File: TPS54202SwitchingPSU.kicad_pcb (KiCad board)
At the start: 2 copper layers, 10 parts, among them CN1 Header_2_pin, CN2 Header_2_pin, U2 TPS54202DDC

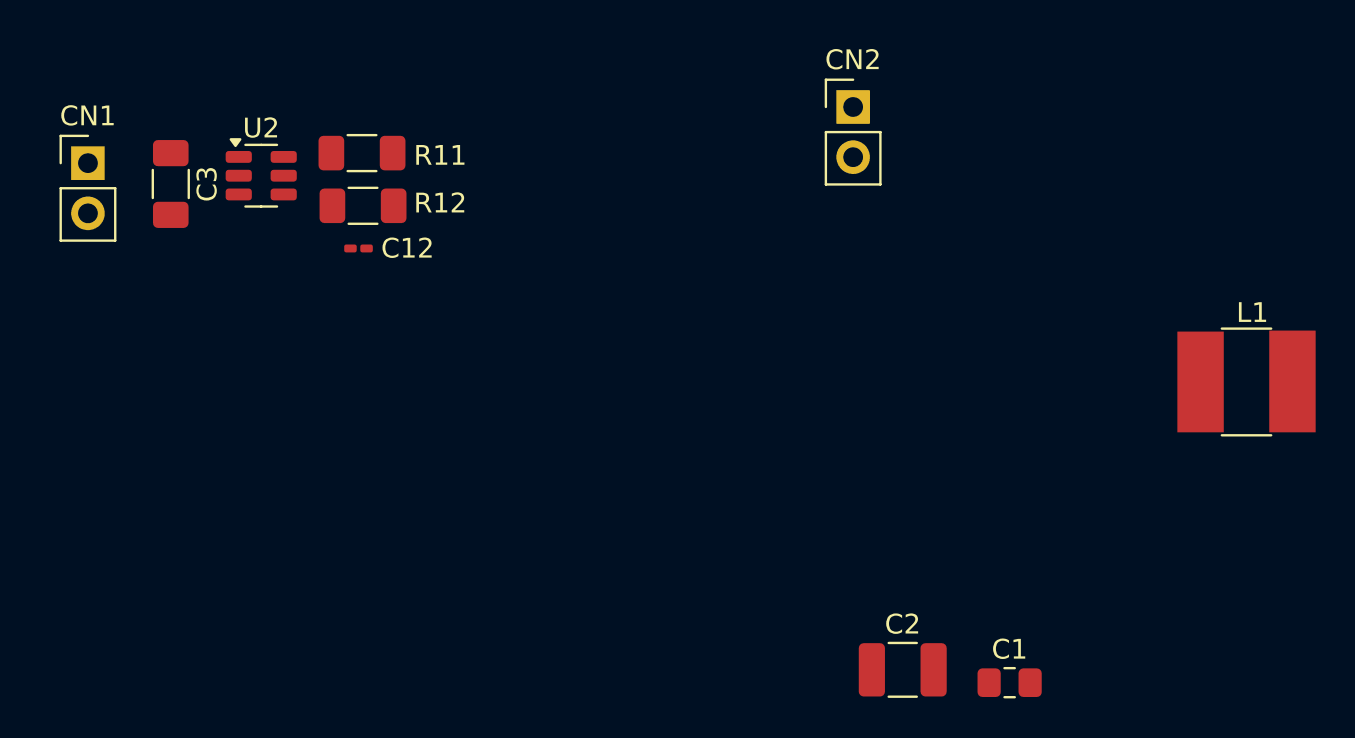
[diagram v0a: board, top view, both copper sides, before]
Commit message: Rev A production release
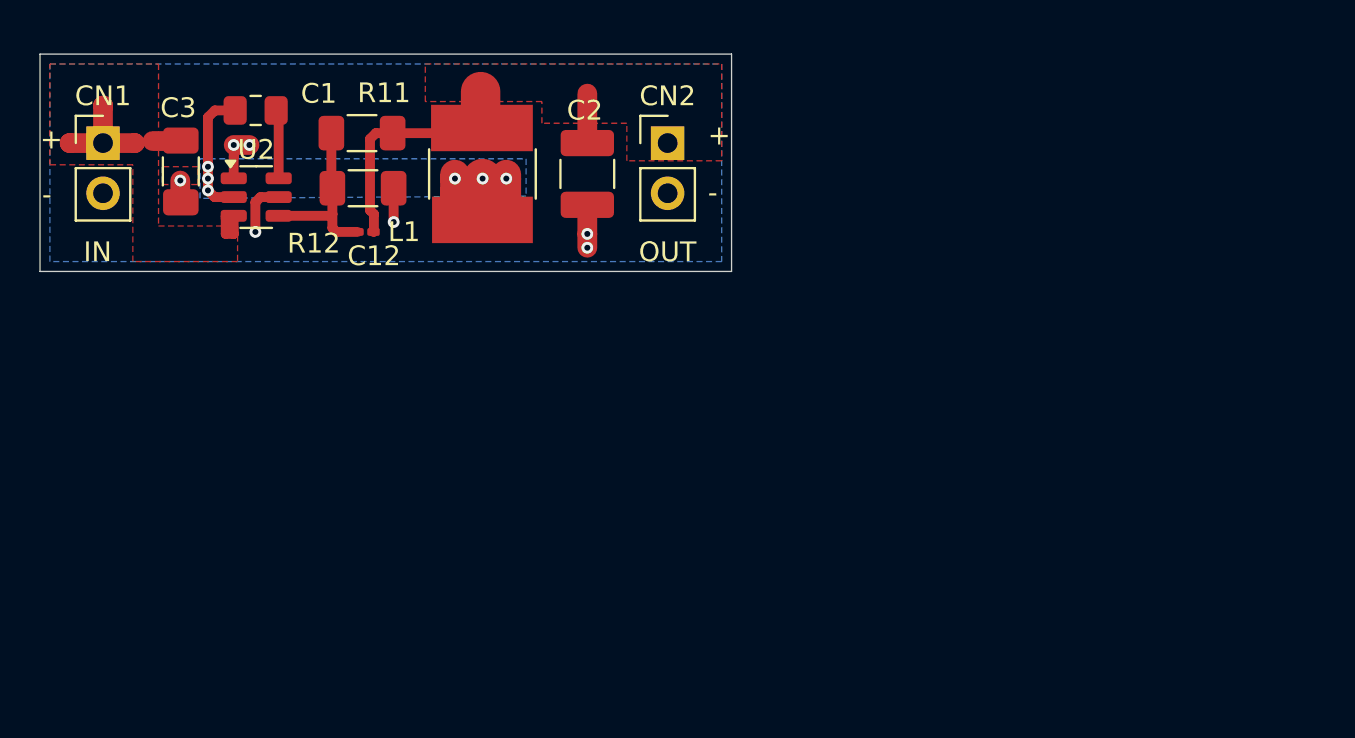
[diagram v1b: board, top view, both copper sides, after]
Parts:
- moved C1 47.9 mm to (122.9, 85.9), turned to 180 degrees
- moved L1 40.1 mm to (134.4, 89.1), turned to 90 degrees
- moved C2 29.7 mm to (139.7, 89.1), turned to -90 degrees
- moved CN2 9.57 mm to (143.8, 87.5)
- moved CN1 1.27 mm to (115.2, 87.5)
- moved U2 1.11 mm to (122.9, 90.2)
- moved R11 1.01 mm to (128.3, 87.0)
- moved C12 0.91 mm to (128.5, 92.0)
- moved R12 0.89 mm to (128.3, 89.8)
- moved C3 0.81 mm to (119.1, 88.9)
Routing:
- net Net-(U2-SW): track 0.00 -> 17.6 mm, vias 0 -> 6
- net /Vout: track 0.00 -> 16.1 mm
- net /Vin: track 0.00 -> 9.06 mm
- net Net-(U2-FB): track 0.00 -> 8.94 mm
- net GND: track 0.00 -> 7.76 mm, vias 0 -> 6
- net Net-(U2-BOOT): track 0.00 -> 3.49 mm
- net unconnected-(U2-EN-Pad5): track 0.00 -> 2.88 mm, vias 0 -> 1
- added copper zone on F.Cu, net /Vin
- added copper zone on F.Cu, net /Vout
- added copper zone on B.Cu, net GND
- added copper zone on F.Cu, net GND
- added copper zone on B.Cu, net Net-(U2-SW)
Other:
- board outline added: 35 x 11 mm
- board text added: "+"
- board text added: "-"
- board text added: "AD Gaming"
- board text added: "IN"
- board text added: "OUT"
- board text added: "Rev A"
- board text added: "TPS54202 PSU"
